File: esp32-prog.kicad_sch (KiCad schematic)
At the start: 14 parts

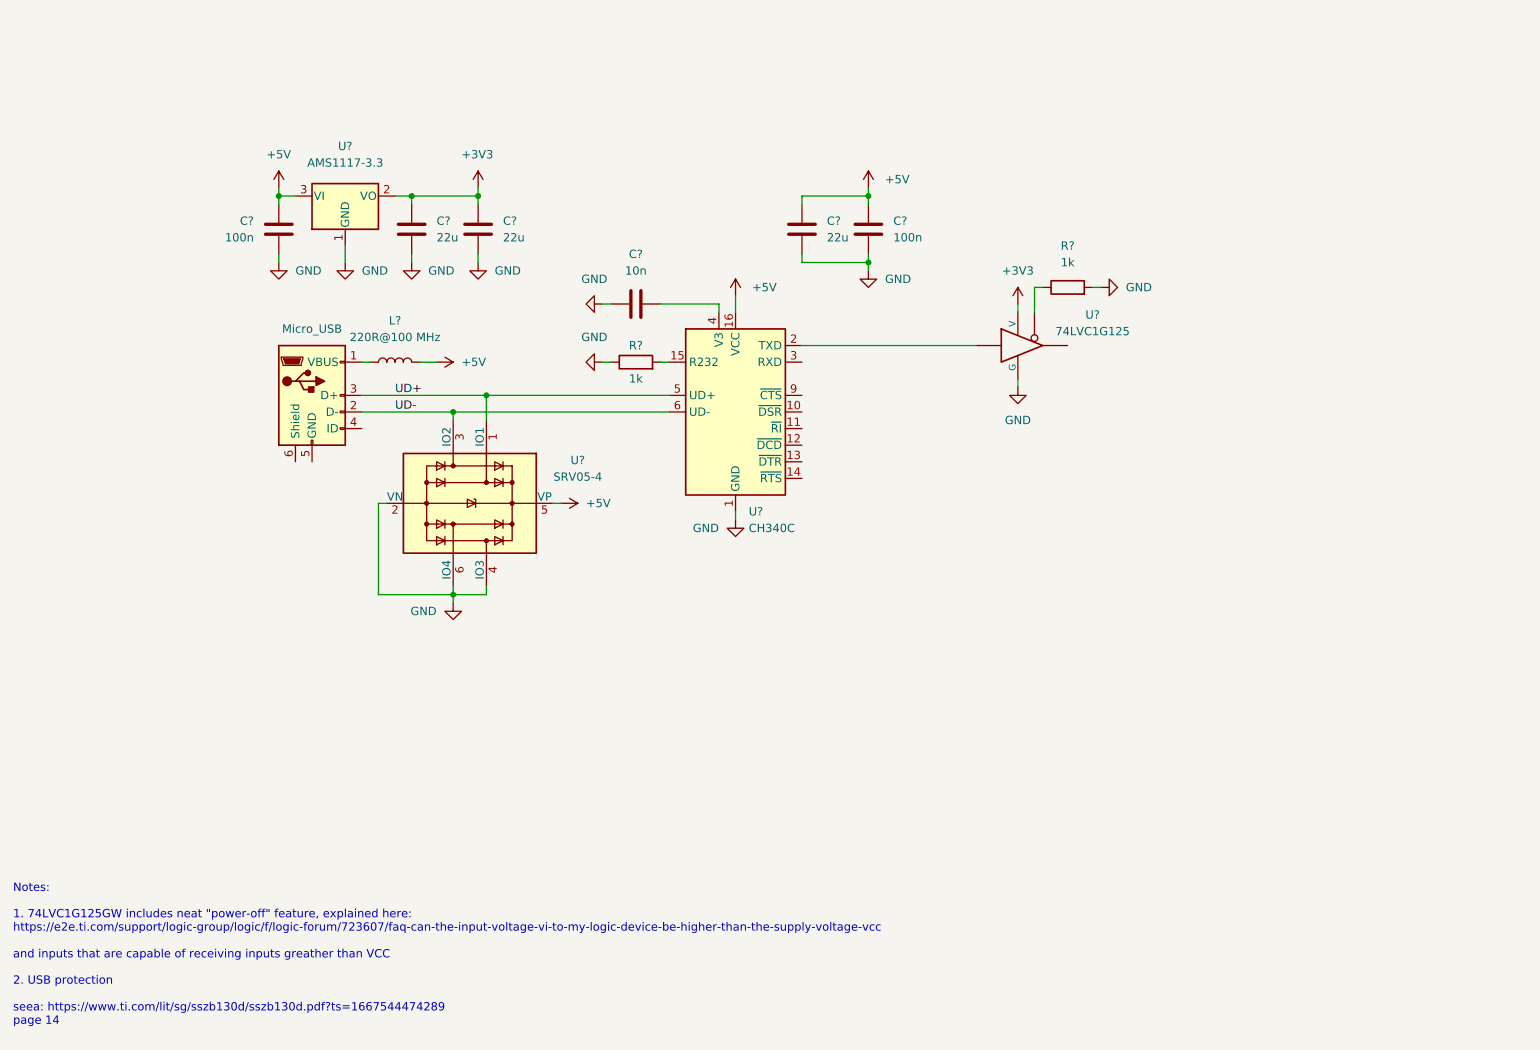
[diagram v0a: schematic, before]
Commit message: draft schematics complete
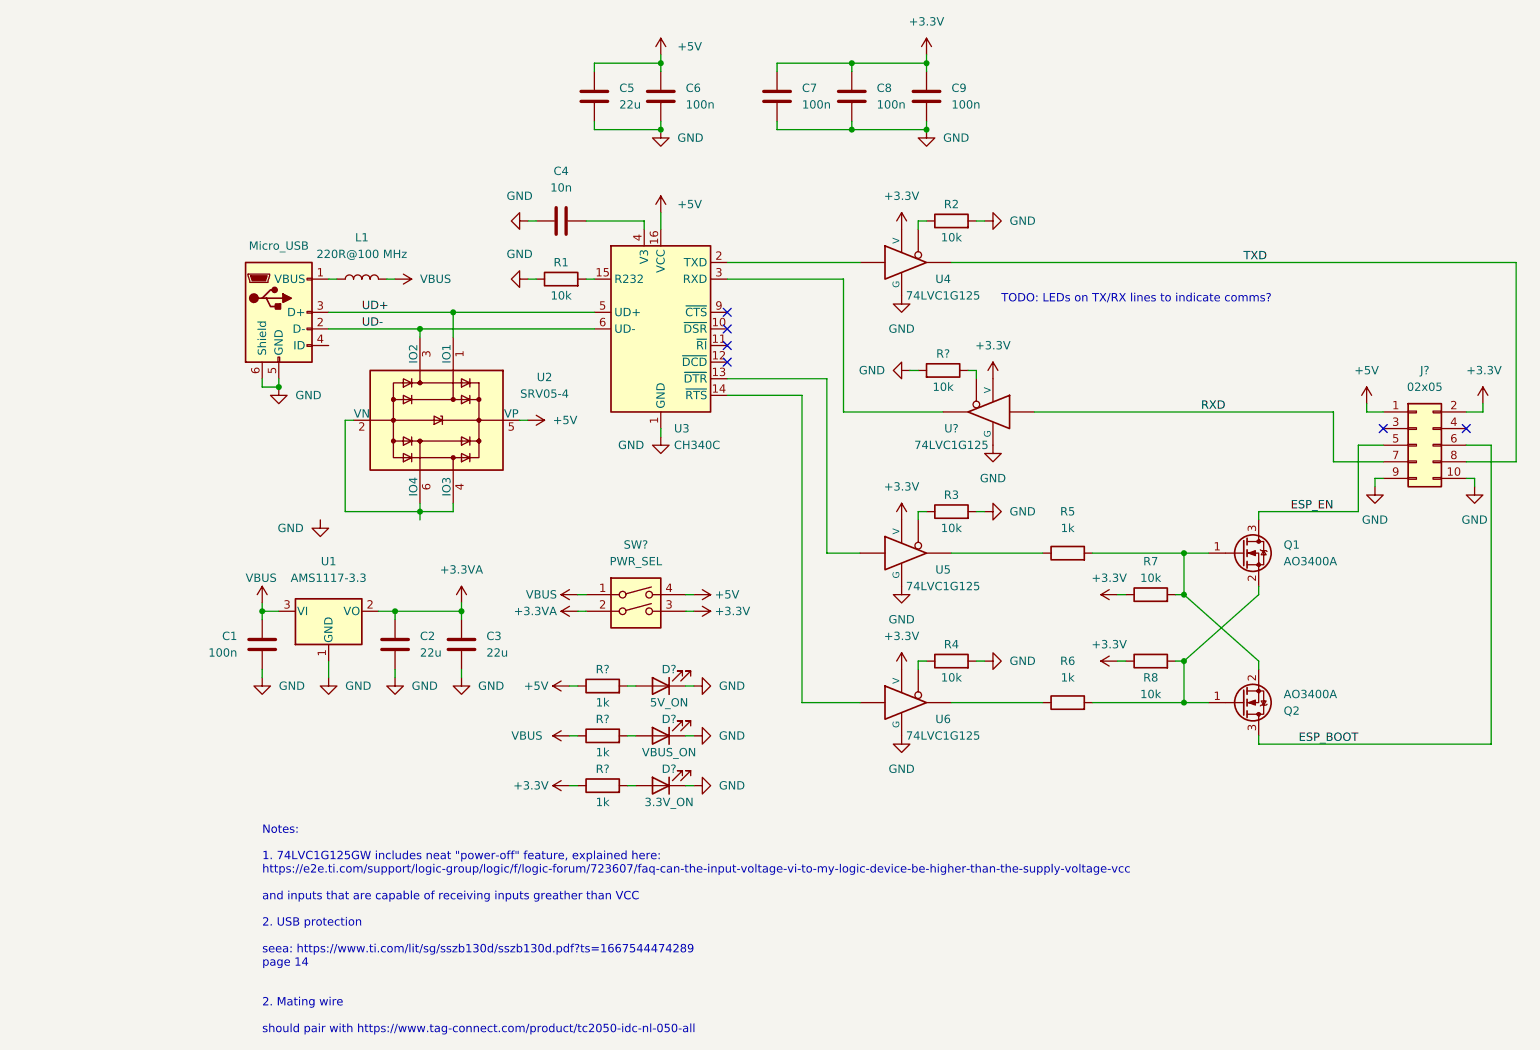
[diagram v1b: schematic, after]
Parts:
- added C7, C8, C9: 100n_0402_CL05B104KB54PNC, Capacitor_SMD:C_0603_1608Metric, symbol 00-kiml-capacitors-smd:100n_0402_CL05B104KB54PNC
- added D? (x3): 0603_RED_KT-0603R, LED_SMD:LED_0603_1608Metric, symbol 00-kiml-led-smd:0603_RED_KT-0603R
- added J?: 1.27mm_50mils_male_DW127R-22-10-23_02x05, Connector_PinHeader_1.27mm:PinHeader_2x05_P1.27mm_Vertical, symbol 00-kiml-connector-pin-header-1.27mm:1.27mm_50mils_male_DW127R-22-10-23_02x05
- added Q1, Q2: AO3400A, Package_TO_SOT_SMD:SOT-23, symbol 00-kiml-transitor-fet:AO3400A
- added R3, R4, R7, R8, R?: 10k_0402_0402WGF1002TCE, Resistor_SMD:R_0402_1005Metric, symbol 00-kiml-resistors-smd:10k_0402_0402WGF1002TCE
- added R5, R6, R? (x3): 1k_0402_0402WGF1001TCE, Resistor_SMD:R_0402_1005Metric, symbol 00-kiml-resistors-smd:1k_0402_0402WGF1001TCE
- added SW?: SW_DIP_x02_50mil_1.27mm_TP-02, symbol 00-kiml-button-switch-smd:SW_DIP_x02_50mil_1.27mm_TP-02
- added U5, U6, U?: 74LVC1G125GW_Nexperia, Package_TO_SOT_SMD:SOT-23-5, symbol 00-kiml-74xGxx:74LVC1G125GW_Nexperia
- R1, R2: renamed from R?; UserValue 1k -> 10k
- gave numbers to parts that had none: 12
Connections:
- net +5V: now also J?.1 (Pin_1), R?.1, SW?.4; no longer C1.1, L1.2, U1.3 (VI)
- net GND: now also J1.5 (GND), J1.6 (Shield), C7.2, C8.2, C9.2, D?.1 (K), D?.1 (K), D?.1 (K), J?.10 (Pin_10), J?.9 (Pin_9), R3.2, R4.2, R?.2, U5.3 (G), U6.3 (G), U?.3 (G); no longer U2.2 (VN), U2.4 (IO3), U2.6 (IO4)
- net TXD: now reaches U4.4
- net TXD: now also J?.8 (Pin_8)
- net at U3.13 (~{DTR}): now also U5.2
- net at U3.14 (~{RTS}): now also U6.2
- net at U3.3 (RXD): now also U?.4
- net +3V3 renamed +3.3VA
- net +3.3VA: now also SW?.2; no longer U4.5 (V)
- new net: Q1.2 (S), Q2.1 (G), R6.2, R8.2
- new net: R6.1, U6.4
- new net: D?.2 (A), R?.2 (x3)
- new net: R5.1, U5.4
- new net: Q1.1 (G), Q2.2 (S), R5.2, R7.2
- new net: R?.1, U?.1
- new net: R4.1, U6.1
- new net: R3.1, U5.1
- new net: U2.2 (VN), U2.4 (IO3), U2.6 (IO4)
- new net +3.3V: C7.1, C8.1, C9.1, J?.2 (Pin_2), R7.1, R8.1, R?.1, SW?.3, U4.5 (V), U5.5 (V), U6.5 (V), U?.5 (V)
- new net ESP_BOOT: J?.6 (Pin_6), Q2.3 (D)
- new net ESP_EN: J?.5 (Pin_5), Q1.3 (D)
- new net RXD: J?.7 (Pin_7), U?.2
- new net VBUS: C1.1, L1.2, R?.1, SW?.1, U1.3 (VI)
- no-connect marks 0 -> 6
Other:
- note added: "2. Mating wire should pair with https://www.tag-connect.com/product/tc2050-idc-nl-050-all"
- note added: "TODO: LEDs on TX/RX lines to indicate comms?"
- moved on the sheet: C1, C2, C3, C4, C5, C6, L1, R1, R2, U1, U2, U3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
